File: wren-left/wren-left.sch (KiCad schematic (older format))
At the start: 65 parts, among them J1 TRRS_Jack, SW0 Reset, U1 ProMicro

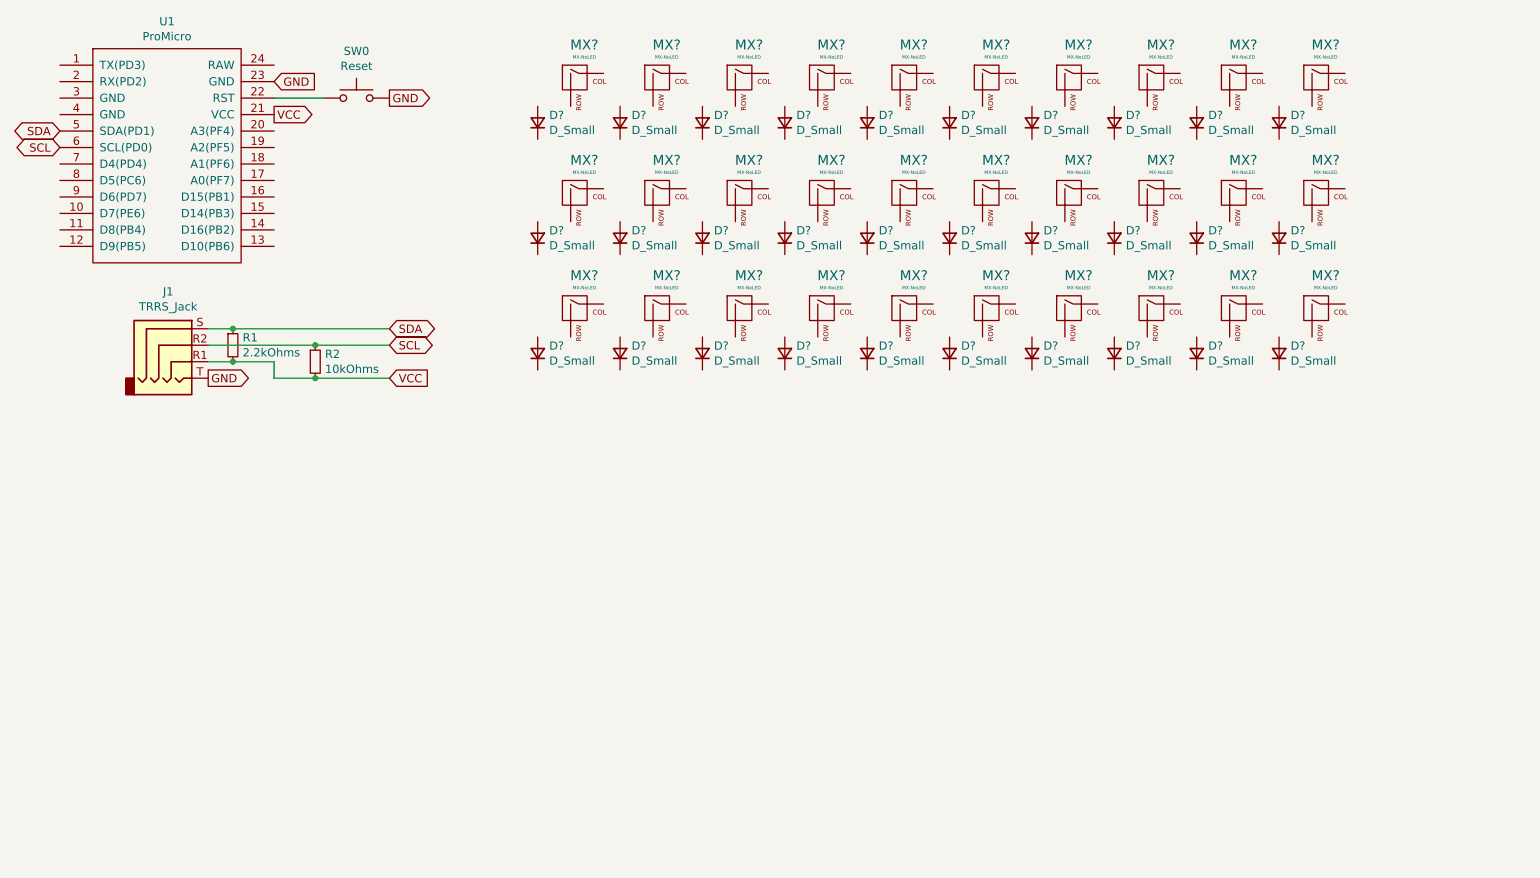
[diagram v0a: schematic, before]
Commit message: Finish Left-Hand Schematic
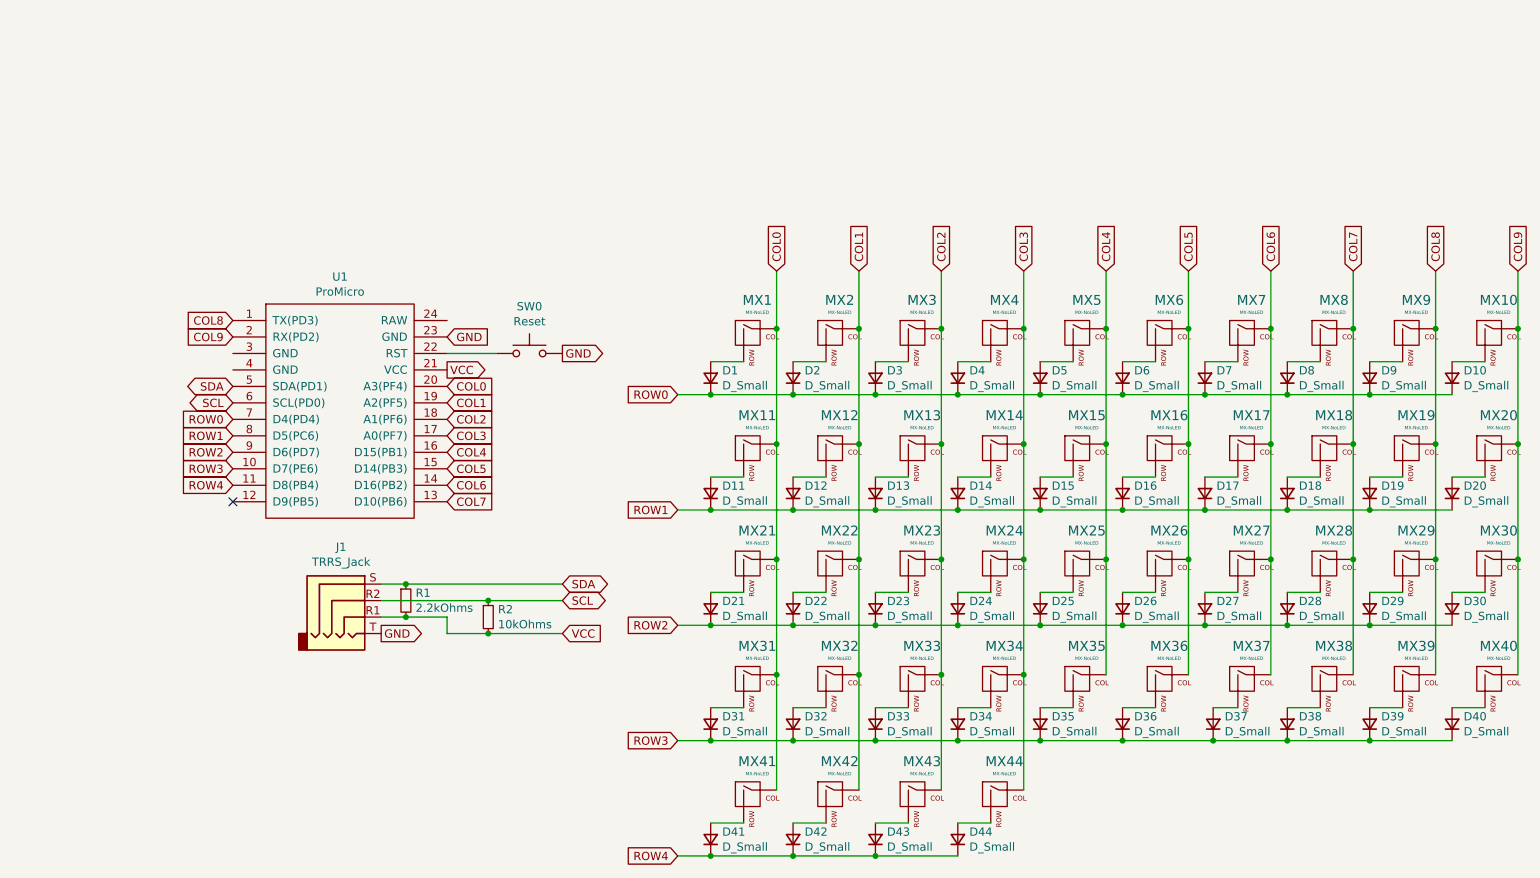
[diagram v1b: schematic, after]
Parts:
- added D31, D32, D33, D34, D35, D36, D37, D38, D39, D40, D41, D42, D43, D44: D_Small, Diode_SMD:D_SOD-123, symbol Device:D_Small
- added MX31, MX32, MX33, MX34, MX35, MX36, MX37, MX38, MX39, MX40, MX42, MX43, MX44: MX-NoLED, MX_Only:MX-1U, symbol MX_Alps_Hybrid:MX-NoLED
- added MX41: MX-NoLED, MX_Only:MX-1.5U, symbol MX_Alps_Hybrid:MX-NoLED
- D1, D10, D11, D12, D13, D14, D15, D16, D17, D18, D19, D2, D20, D21, D22, D23, D24, D25, D26, D27, D28, D29, D3, D30, D4, D5, D6, D7, D8, D9: renamed from D?; footprint (none) -> Diode_SMD:D_SOD-123
- J1: footprint (none) -> footprints:TRRS_JACK_MJ4PP9
- MX1, MX10, MX11, MX12, MX13, MX14, MX15, MX16, MX17, MX18, MX19, MX2, MX20, MX21, MX22, MX23, MX24, MX25, MX26, MX27, MX28, MX29, MX3, MX30, MX4, MX5, MX6, MX7, MX8, MX9: renamed from MX?; footprint (none) -> MX_Only:MX-1U
- R1, R2: footprint (none) -> Resistor_SMD:R_0805_2012Metric
- SW0: footprint (none) -> random-keyboard-parts:SKQG-1155865
- U1: footprint (none) -> footprints:ARDUINO_PRO_MICRO
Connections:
- net COL8: now reaches U1.1 (TX(PD3))
- net COL8: now also MX19.1 (COL), MX29.1 (COL), MX9.1 (COL), MX39.1 (COL)
- net ROW3: now reaches U1.10 (D7(PE6))
- net ROW3: now also D31.1 (K), D32.1 (K), D33.1 (K), D34.1 (K), D35.1 (K), D36.1 (K), D37.1 (K), D38.1 (K), D39.1 (K), D40.1 (K)
- net ROW4: now reaches U1.11 (D8(PB4))
- net ROW4: now also D41.1 (K), D42.1 (K), D43.1 (K), D44.1 (K)
- net COL7: now reaches U1.13 (D10(PB6))
- net COL7: now also MX18.1 (COL), MX28.1 (COL), MX8.1 (COL), MX38.1 (COL)
- net COL6: now reaches U1.14 (D16(PB2))
- net COL6: now also MX17.1 (COL), MX27.1 (COL), MX7.1 (COL), MX37.1 (COL)
- net COL5: now reaches U1.15 (D14(PB3))
- net COL5: now also MX16.1 (COL), MX26.1 (COL), MX6.1 (COL), MX36.1 (COL)
- net COL4: now reaches U1.16 (D15(PB1))
- net COL4: now also MX15.1 (COL), MX25.1 (COL), MX5.1 (COL), MX35.1 (COL)
- net COL3: now reaches U1.17 (A0(PF7))
- net COL3: now also MX14.1 (COL), MX24.1 (COL), MX4.1 (COL), MX34.1 (COL), MX44.1 (COL)
- net COL2: now reaches U1.18 (A1(PF6))
- net COL2: now also MX13.1 (COL), MX23.1 (COL), MX3.1 (COL), MX33.1 (COL), MX43.1 (COL)
- net COL1: now reaches U1.19 (A2(PF5))
- net COL1: now also MX12.1 (COL), MX2.1 (COL), MX22.1 (COL), MX32.1 (COL), MX42.1 (COL)
- net COL9: now reaches U1.2 (RX(PD2))
- net COL9: now also MX10.1 (COL), MX20.1 (COL), MX30.1 (COL), MX40.1 (COL)
- net COL0: now reaches U1.20 (A3(PF4))
- net COL0: now also MX1.1 (COL), MX11.1 (COL), MX21.1 (COL), MX31.1 (COL), MX41.1 (COL)
- net ROW0: now reaches U1.7 (D4(PD4))
- net ROW0: now also D1.1 (K), D10.1 (K), D2.1 (K), D3.1 (K), D4.1 (K), D5.1 (K), D6.1 (K), D7.1 (K), D8.1 (K), D9.1 (K)
- net ROW1: now reaches U1.8 (D5(PC6))
- net ROW1: now also D11.1 (K), D12.1 (K), D13.1 (K), D14.1 (K), D15.1 (K), D16.1 (K), D17.1 (K), D18.1 (K), D19.1 (K), D20.1 (K)
- net ROW2: now reaches U1.9 (D6(PD7))
- net ROW2: now also D21.1 (K), D22.1 (K), D23.1 (K), D24.1 (K), D25.1 (K), D26.1 (K), D27.1 (K), D28.1 (K), D29.1 (K), D30.1 (K)
- net at MX1.2 (ROW): now also D1.2 (A)
- net at MX2.2 (ROW): now also D2.2 (A)
- net at D3.2 (A): now also MX3.2 (ROW)
- net at D4.2 (A): now also MX4.2 (ROW)
- net at D5.2 (A): now also MX5.2 (ROW)
- net at D6.2 (A): now also MX6.2 (ROW)
- net at D7.2 (A): now also MX7.2 (ROW)
- net at D8.2 (A): now also MX8.2 (ROW)
- net at D9.2 (A): now also MX9.2 (ROW)
- net at MX10.2 (ROW): now also D10.2 (A)
- net at MX11.2 (ROW): now also D11.2 (A)
- net at MX12.2 (ROW): now also D12.2 (A)
- net at MX13.2 (ROW): now also D13.2 (A)
- net at MX14.2 (ROW): now also D14.2 (A)
- net at MX15.2 (ROW): now also D15.2 (A)
- net at MX16.2 (ROW): now also D16.2 (A)
- net at MX17.2 (ROW): now also D17.2 (A)
- net at MX18.2 (ROW): now also D18.2 (A)
- net at MX19.2 (ROW): now also D19.2 (A)
- net at MX20.2 (ROW): now also D20.2 (A)
- net at MX21.2 (ROW): now also D21.2 (A)
- net at MX22.2 (ROW): now also D22.2 (A)
- net at MX23.2 (ROW): now also D23.2 (A)
- net at MX24.2 (ROW): now also D24.2 (A)
- net at MX25.2 (ROW): now also D25.2 (A)
- net at MX26.2 (ROW): now also D26.2 (A)
- net at MX27.2 (ROW): now also D27.2 (A)
- net at MX28.2 (ROW): now also D28.2 (A)
- net at MX29.2 (ROW): now also D29.2 (A)
- net at MX30.2 (ROW): now also D30.2 (A)
- new net: D31.2 (A), MX31.2 (ROW)
- new net: D32.2 (A), MX32.2 (ROW)
- new net: D33.2 (A), MX33.2 (ROW)
- new net: D34.2 (A), MX34.2 (ROW)
- new net: D35.2 (A), MX35.2 (ROW)
- new net: D36.2 (A), MX36.2 (ROW)
- new net: D37.2 (A), MX37.2 (ROW)
- new net: D38.2 (A), MX38.2 (ROW)
- new net: D39.2 (A), MX39.2 (ROW)
- new net: D40.2 (A), MX40.2 (ROW)
- new net: D41.2 (A), MX41.2 (ROW)
- new net: D42.2 (A), MX42.2 (ROW)
- new net: D43.2 (A), MX43.2 (ROW)
- new net: D44.2 (A), MX44.2 (ROW)
- no-connect marks 0 -> 1
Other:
- moved on the sheet: D1, D10, D11, D12, D13, D14, D15, D16, D17, D18, D19, D2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

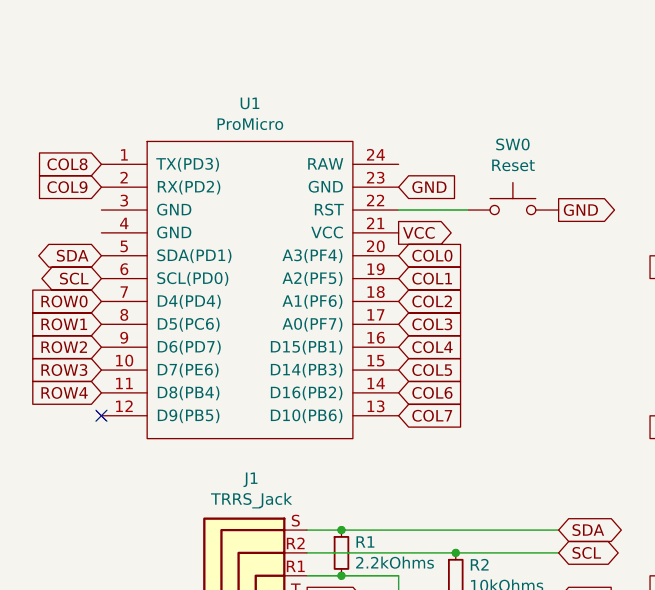
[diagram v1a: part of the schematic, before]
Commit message: Routing Half-Finished
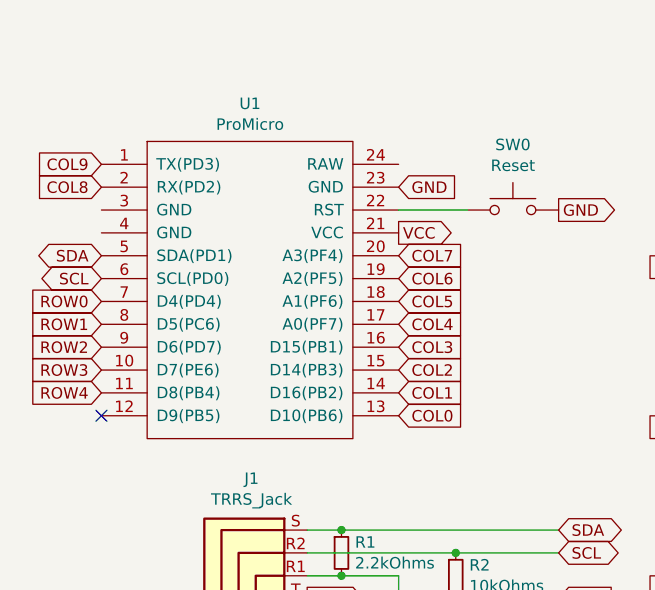
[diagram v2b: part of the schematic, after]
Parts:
- J1: footprint footprints:TRRS_JACK_MJ4PP9 -> Connector_Audio:Jack_3.5mm_PJ320E_Horizontal
- MX41: footprint MX_Only:MX-1.5U -> MX_Only:MX-2U-FLIPPED-ReversedStabilizers
- SW0: footprint random-keyboard-parts:SKQG-1155865 -> Button_Switch_THT:SW_PUSH_6mm
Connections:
- net COL0: now also U1.13 (D10(PB6)); no longer U1.20 (A3(PF4))
- net COL1: now also U1.14 (D16(PB2)); no longer U1.19 (A2(PF5))
- net COL2: now also U1.15 (D14(PB3)); no longer U1.18 (A1(PF6))
- net COL3: now also U1.16 (D15(PB1)); no longer U1.17 (A0(PF7))
- net COL4: now also U1.17 (A0(PF7)); no longer U1.16 (D15(PB1))
- net COL5: now also U1.18 (A1(PF6)); no longer U1.15 (D14(PB3))
- net COL6: now also U1.19 (A2(PF5)); no longer U1.14 (D16(PB2))
- net COL7: now also U1.20 (A3(PF4)); no longer U1.13 (D10(PB6))
- net COL8: now also U1.2 (RX(PD2)); no longer U1.1 (TX(PD3))
- net COL9: now also U1.1 (TX(PD3)); no longer U1.2 (RX(PD2))
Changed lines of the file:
@@
 F 0 "J1" H 2607 4675 50  0000 C CNN
 F 1 "TRRS_Jack" H 2607 4584 50  0000 C CNN
-F 2 "footprints:TRRS_JACK_MJ4PP9" H 2650 4350 50  0001 C CNN
+F 2 "Connector_Audio:Jack_3.5mm_PJ320E_Horizontal" H 2650 4350 50  0001 C CNN
 F 3 "~" H 2650 4350 50  0001 C CNN
 	1    2650 4350
@@
 F 0 "SW0" H 3750 3135 50  0000 C CNN
 F 1 "Reset" H 3750 3044 50  0000 C CNN
-F 2 "random-keyboard-parts:SKQG-1155865" H 3750 3050 50  0001 C CNN
+F 2 "Button_Switch_THT:SW_PUSH_6mm" H 3750 3050 50  0001 C CNN
 F 3 "~" H 3750 3050 50  0001 C CNN
 	1    3750 2850
@@
 F 0 "MX41" H 5133 5773 60  0000 C CNN
 F 1 "MX-NoLED" H 5133 5699 20  0000 C CNN
-F 2 "MX_Only:MX-1.5U" H 4475 5525 60  0001 C CNN
+F 2 "MX_Only:MX-2U-FLIPPED-ReversedStabilizers" H 4475 5525 60  0001 C CNN
 F 3 "" H 4475 5525 60  0001 C CNN
 	1    5100 5550
@@
 Text GLabel 9750 2350 1    50   Input ~ 0
 COL9
+Text GLabel 3250 3750 2    50   Input ~ 0
+COL0
+Text GLabel 3250 3650 2    50   Input ~ 0
+COL1
+Text GLabel 3250 3550 2    50   Input ~ 0
+COL2
+Text GLabel 3250 3450 2    50   Input ~ 0
+COL3
+Text GLabel 3250 3350 2    50   Input ~ 0
+COL4
+Text GLabel 3250 3250 2    50   Input ~ 0
+COL5
+Text GLabel 3250 3150 2    50   Input ~ 0
+COL6
 Text GLabel 3250 3050 2    50   Input ~ 0
-COL0
-Text GLabel 3250 3150 2    50   Input ~ 0
-COL1
-Text GLabel 3250 3250 2    50   Input ~ 0
-COL2
-Text GLabel 3250 3350 2    50   Input ~ 0
-COL3
-Text GLabel 3250 3450 2    50   Input ~ 0
-COL4
-Text GLabel 3250 3550 2    50   Input ~ 0
-COL5
-Text GLabel 3250 3650 2    50   Input ~ 0
-COL6
-Text GLabel 3250 3750 2    50   Input ~ 0
 COL7
+Text GLabel 1950 2750 0    50   Input ~ 0
+COL8
 Text GLabel 1950 2650 0    50   Input ~ 0
-COL8
-Text GLabel 1950 2750 0    50   Input ~ 0
 COL9
 Text GLabel 1950 3250 0    50   Input ~ 0
